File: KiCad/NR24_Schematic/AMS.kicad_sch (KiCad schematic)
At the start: 4 parts

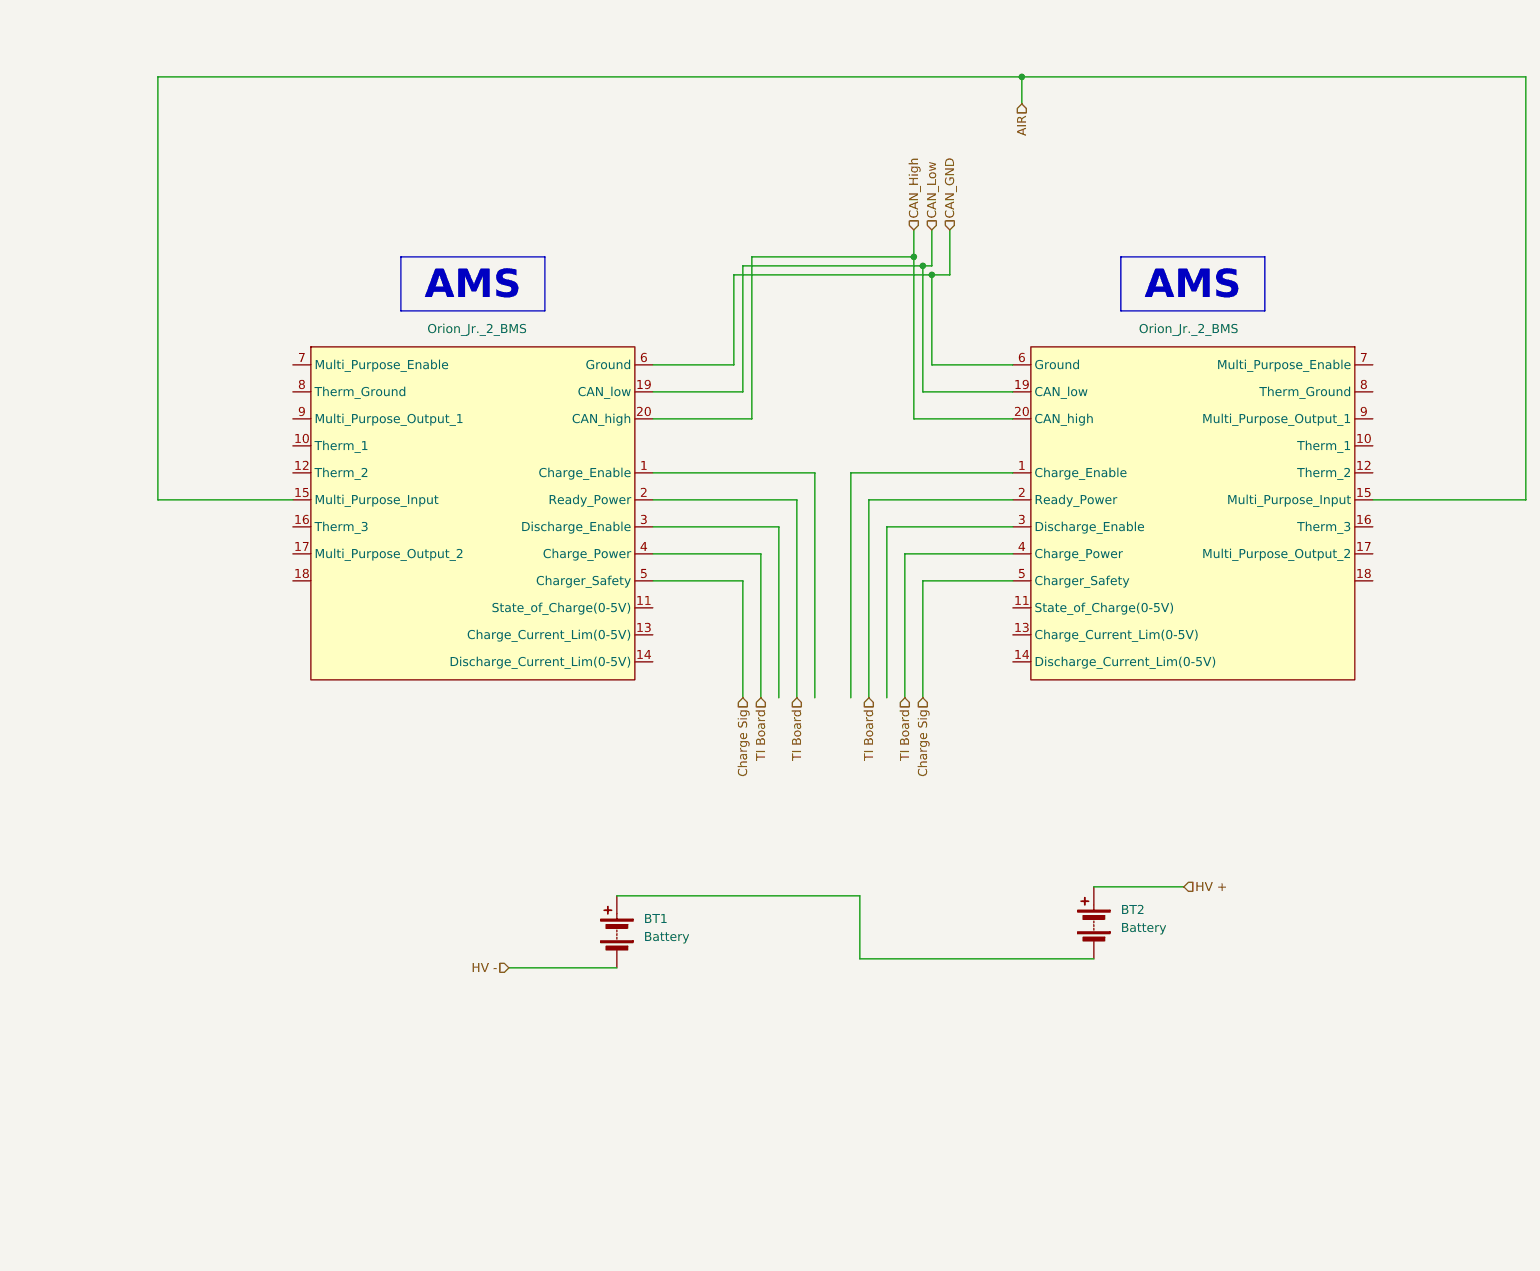
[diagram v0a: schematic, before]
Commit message: uh
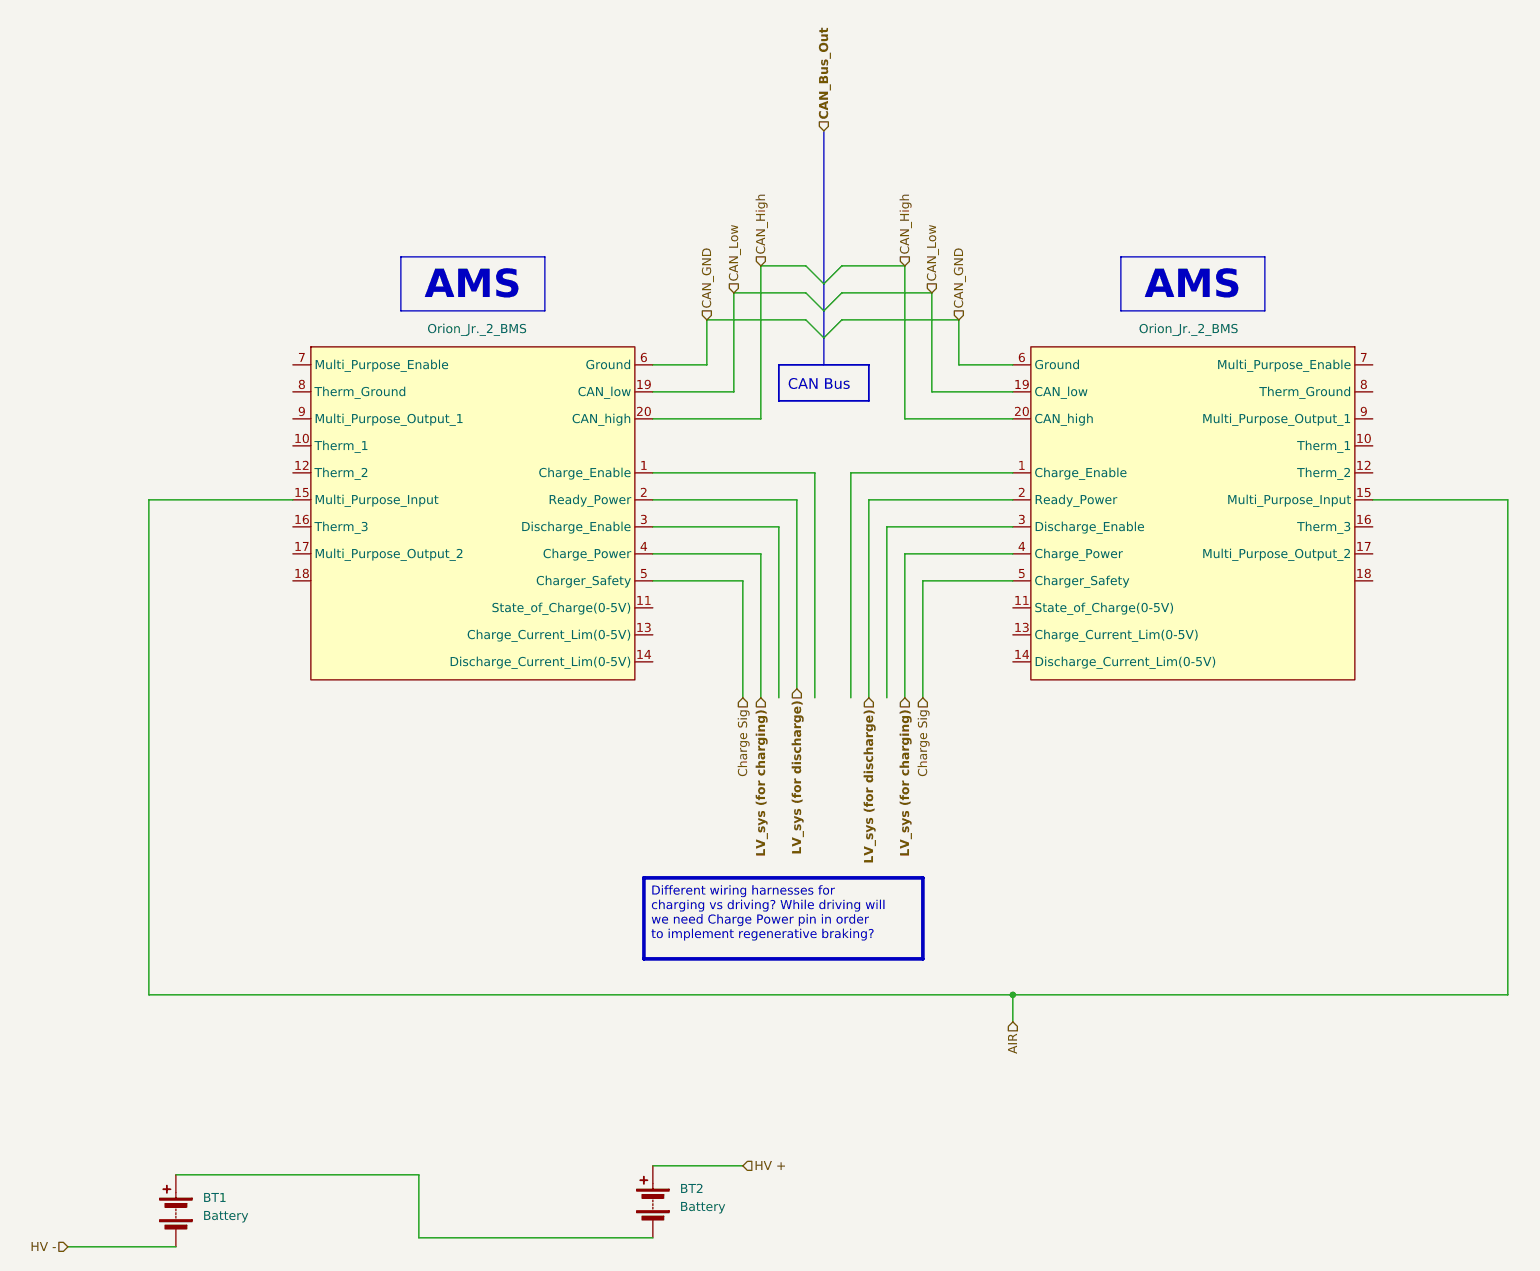
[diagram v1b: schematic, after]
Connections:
- net TI Board renamed LV_sys (for charging)
- net LV_sys (for charging): no longer U?.2 (Ready_Power), U?.2 (Ready_Power)
- new net LV_sys (for discharge): U?.2 (Ready_Power), U?.2 (Ready_Power)
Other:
- note added: "CAN Bus"
- moved on the sheet: BT1, BT2
